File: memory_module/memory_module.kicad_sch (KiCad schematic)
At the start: 93 parts, among them J1 Conn_01x06_Pin, J2 Conn_01x08_Pin, SW1 SW_DIP_x08, SW2 SW_DIP_x08, SW3 SW_DIP_x08, SW4 SW_DIP_x08, SW5 SW_DIP_x08, SW6 SW_DIP_x08, SW7 SW_DIP_x08, SW8 SW_DIP_x08, U1 74HC138, U2 74HC540

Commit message: wip
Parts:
- added D100, D101, D102, D103, D104, D105, D106, D107, D108, D109, D110, D111, D112, D113, D114, D115, D116, D117, D118, D119, D120, D121, D122, D123, D124, D125, D126, D127, D128, D65, D66, D67, D68, D69, D70, D71, D72, D73, D74, D75, D76, D77, D78, D79, D80, D81, D82, D83, D84, D85, D86, D87, D88, D89, D90, D91, D92, D93, D94, D95, D96, D97, D98, D99: 1N4148, Diode_THT:D_DO-35_SOD27_P2.54mm_Vertical_KathodeUp, symbol Diode:1N4148
- added D137, D138, D139, D140, D141, D142, D143, D144: LED, LED_THT:LED_D3.0mm, symbol Device:LED
- added SW10, SW11, SW12, SW13, SW14, SW15, SW16, SW9: SW_DIP_x08, Button_Switch_THT:SW_DIP_SPSTx08_Slide_9.78x22.5mm_W7.62mm_P2.54mm, symbol Switch:SW_DIP_x08
- added U2: 74HC138, TD4_footprint:DIP16_TOS, symbol 74xx:74HC138
- D1, D10, D11, D12, D13, D14, D15, D16, D17, D18, D19, D2, D20, D21, D22, D23, D24, D25, D26, D27, D28, D29, D3, D30, D31, D32, D33, D34, D35, D36, D37, D38, D39, D4, D40, D41, D42, D43, D44, D45, D46, D47, D48, D49, D5, D50, D51, D52, D53, D54, D55, D56, D57, D58, D59, D6, D60, D61, D62, D63, D64, D7, D8, D9: footprint Diode_THT:D_DO-35_SOD27_P7.62mm_Horizontal -> Diode_THT:D_DO-35_SOD27_P2.54mm_Vertical_KathodeUp
- renumbered D65 to D129, D66 to D130, D67 to D131, D68 to D132, D69 to D133, D70 to D134, D71 to D135, D72 to D136, U2 to U3
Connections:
- net +5V: now also U2.16 (VCC)
- net A0: now also U2.1 (A0)
- net A1: now also U2.2 (A1)
- net A2: now also U2.3 (A2)
- net GND: now also U2.5 (~{E1}), U2.6 (E2), U2.8 (GND); no longer J1.4 (Pin_4), U1.5 (~{E1}), U1.6 (E2)
- net at D129.2 (A), D130.2 (A), D131.2 (A)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: now also D137.2 (A), D138.2 (A), D139.2 (A), D140.2 (A), D141.2 (A), D142.2 (A), D143.2 (A), D144.2 (A)
- net at R1.1, SW1.16, SW2.16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: now also SW10.16, SW11.16, SW12.16, SW13.16, SW14.16, SW15.16, SW16.16, SW9.16
- net at R3.1, SW1.14, SW2.14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: now also SW10.14, SW11.14, SW12.14, SW13.14, SW14.14, SW15.14, SW16.14, SW9.14
- net at R6.1, SW1.11, SW2.11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: now also SW10.11, SW11.11, SW12.11, SW13.11, SW14.11, SW15.11, SW16.11, SW9.11
- net at R2.1, SW1.15, SW2.15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: now also SW10.15, SW11.15, SW12.15, SW13.15, SW14.15, SW15.15, SW16.15, SW9.15
- net at R7.1, SW1.10, SW2.10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: now also SW10.10, SW11.10, SW12.10, SW13.10, SW14.10, SW15.10, SW16.10, SW9.10
- net at R5.1, SW1.12, SW2.12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: now also SW10.12, SW11.12, SW12.12, SW13.12, SW14.12, SW15.12, SW16.12, SW9.12
- net at R4.1, SW1.13, SW2.13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: now also SW10.13, SW11.13, SW12.13, SW13.13, SW14.13, SW15.13, SW16.13, SW9.13
- net at R8.1, SW1.9, SW2.9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: now also SW10.9, SW11.9, SW12.9, SW13.9, SW14.9, SW15.9, SW16.9, SW9.9
- new net: D100.1 (K), D101.1 (K), D102.1 (K), D103.1 (K), D104.1 (K), D97.1 (K), D98.1 (K), D99.1 (K)
- new net: D98.2 (A), SW13.2
- new net: D121.2 (A), SW16.1
- new net: D122.2 (A), SW16.2
- new net: D123.2 (A), SW16.3
- new net: D124.2 (A), SW16.4
- new net: D125.2 (A), SW16.5
- new net: D126.2 (A), SW16.6
- new net: D127.2 (A), SW16.7
- new net: D128.2 (A), SW16.8
- new net: D73.1 (K), D74.1 (K), D75.1 (K), D76.1 (K), D77.1 (K), D78.1 (K), D79.1 (K), D80.1 (K)
- new net: D74.2 (A), SW10.2
- new net: D105.1 (K), D106.1 (K), D107.1 (K), D108.1 (K), D109.1 (K), D110.1 (K), D111.1 (K), D112.1 (K)
- new net: D112.2 (A), SW14.8
- new net: D78.2 (A), SW10.6
- new net: D65.2 (A), SW9.1
- new net: D66.2 (A), SW9.2
- new net: D67.2 (A), SW9.3
- new net: D68.2 (A), SW9.4
- new net: D69.2 (A), SW9.5
- new net: D70.2 (A), SW9.6
- new net: D71.2 (A), SW9.7
- new net: D72.2 (A), SW9.8
- new net: D65.1 (K), D66.1 (K), D67.1 (K), D68.1 (K), D69.1 (K), D70.1 (K), D71.1 (K), D72.1 (K)
- new net: D75.2 (A), SW10.3
- new net: D138.1 (K), U2.14 (~{Y1})
- new net: D121.1 (K), D122.1 (K), D123.1 (K), D124.1 (K), D125.1 (K), D126.1 (K), D127.1 (K), D128.1 (K)
- new net: D141.1 (K), U2.11 (~{Y4})
- new net: D73.2 (A), SW10.1
- new net: D113.1 (K), D114.1 (K), D115.1 (K), D116.1 (K), D117.1 (K), D118.1 (K), D119.1 (K), D120.1 (K)
- new net: D114.2 (A), SW15.2
- new net: D120.2 (A), SW15.8
- new net: D81.1 (K), D82.1 (K), D83.1 (K), D84.1 (K), D85.1 (K), D86.1 (K), D87.1 (K), D88.1 (K)
- new net: D85.2 (A), SW11.5
- new net: D101.2 (A), SW13.5
- new net: D84.2 (A), SW11.4
- new net: D89.1 (K), D90.1 (K), D91.1 (K), D92.1 (K), D93.1 (K), D94.1 (K), D95.1 (K), D96.1 (K)
- new net: D90.2 (A), SW12.2
- new net: D81.2 (A), SW11.1
- new net: D82.2 (A), SW11.2
- new net: D83.2 (A), SW11.3
- new net: D86.2 (A), SW11.6
- new net: D87.2 (A), SW11.7
- new net: D88.2 (A), SW11.8
- new net: D108.2 (A), SW14.4
- new net: D117.2 (A), SW15.5
- new net: D95.2 (A), SW12.7
- new net: D111.2 (A), SW14.7
- new net: D103.2 (A), SW13.7
- new net: D107.2 (A), SW14.3
- new net: D105.2 (A), SW14.1
- new net: D106.2 (A), SW14.2
- new net: D109.2 (A), SW14.5
- new net: D110.2 (A), SW14.6
- new net: D139.1 (K), U2.13 (~{Y2})
- new net: D91.2 (A), SW12.3
- new net: D119.2 (A), SW15.7
- new net: D77.2 (A), SW10.5
- new net: D93.2 (A), SW12.5
- new net: D97.2 (A), SW13.1
- new net: D99.2 (A), SW13.3
- new net: D100.2 (A), SW13.4
- new net: D102.2 (A), SW13.6
- new net: D104.2 (A), SW13.8
- new net: D137.1 (K), U2.15 (~{Y0})
- new net: D144.1 (K), U2.7 (~{Y7})
- new net: D115.2 (A), SW15.3
- new net: D89.2 (A), SW12.1
- new net: D92.2 (A), SW12.4
- new net: D94.2 (A), SW12.6
- new net: D96.2 (A), SW12.8
- new net: D142.1 (K), U2.10 (~{Y5})
- new net: D140.1 (K), U2.12 (~{Y3})
- new net: D143.1 (K), U2.9 (~{Y6})
- new net: D76.2 (A), SW10.4
- new net: D113.2 (A), SW15.1
- new net: D116.2 (A), SW15.4
- new net: D118.2 (A), SW15.6
- new net: D79.2 (A), SW10.7
- new net: D80.2 (A), SW10.8
- new net A3: J1.4 (Pin_4), U1.5 (~{E1}), U1.6 (E2), U2.4 (~{E0})
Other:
- moved on the sheet: D1, D10, D11, D12, D129, D13, D130, D131, D132, D133, D134, D135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

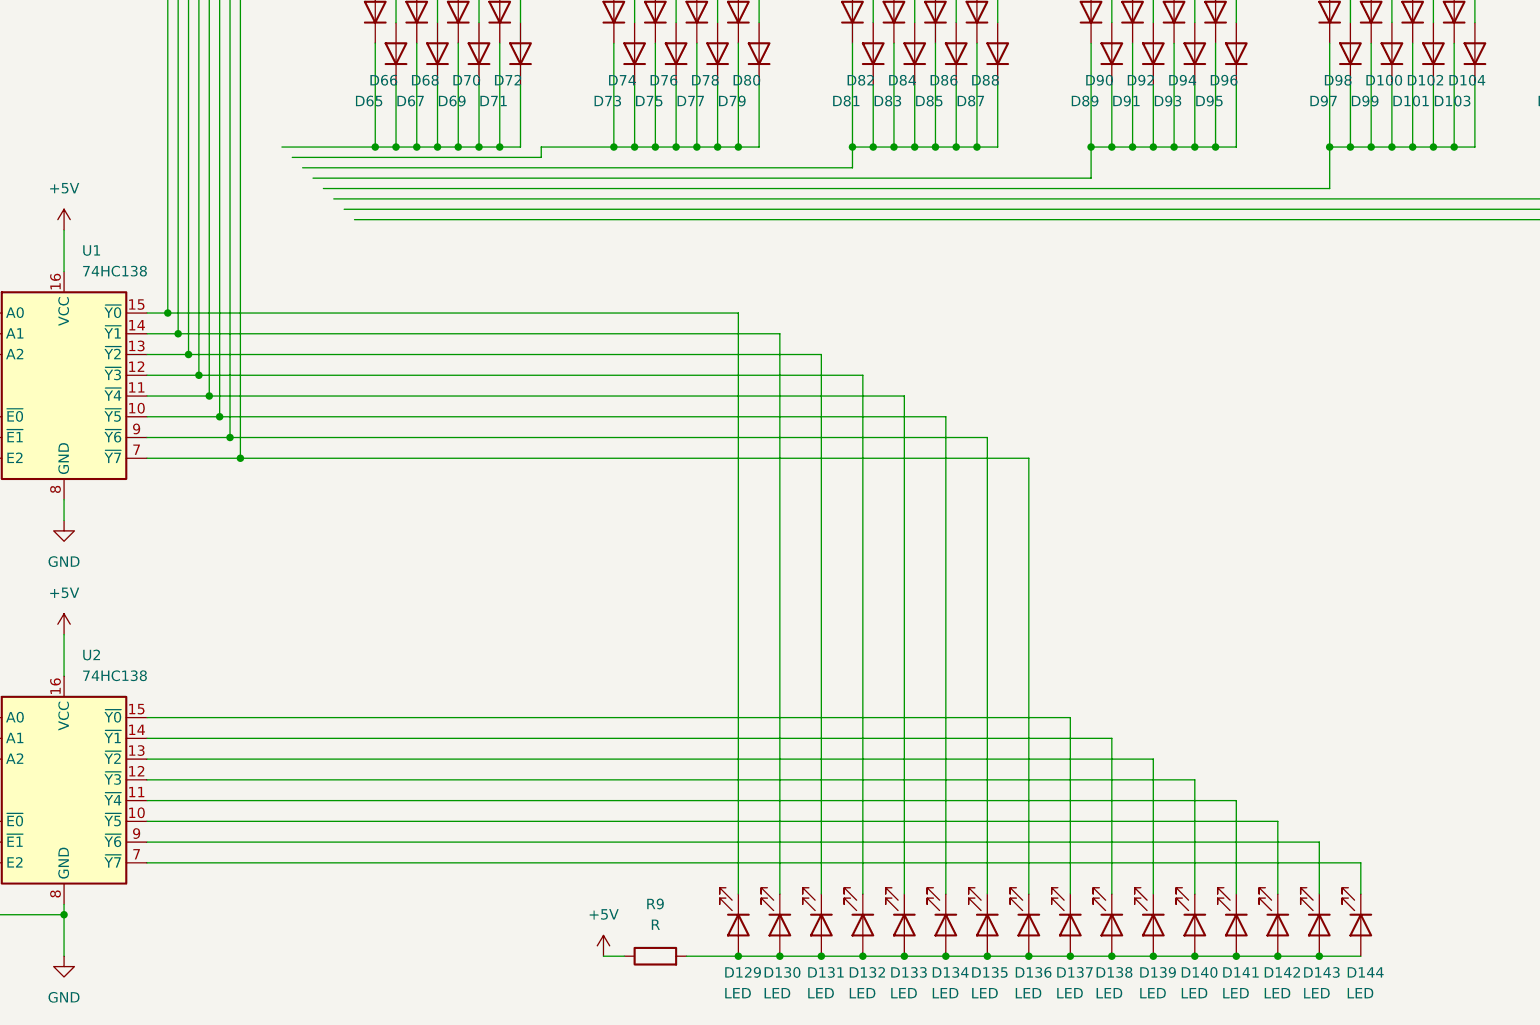
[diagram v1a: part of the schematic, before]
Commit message: wip
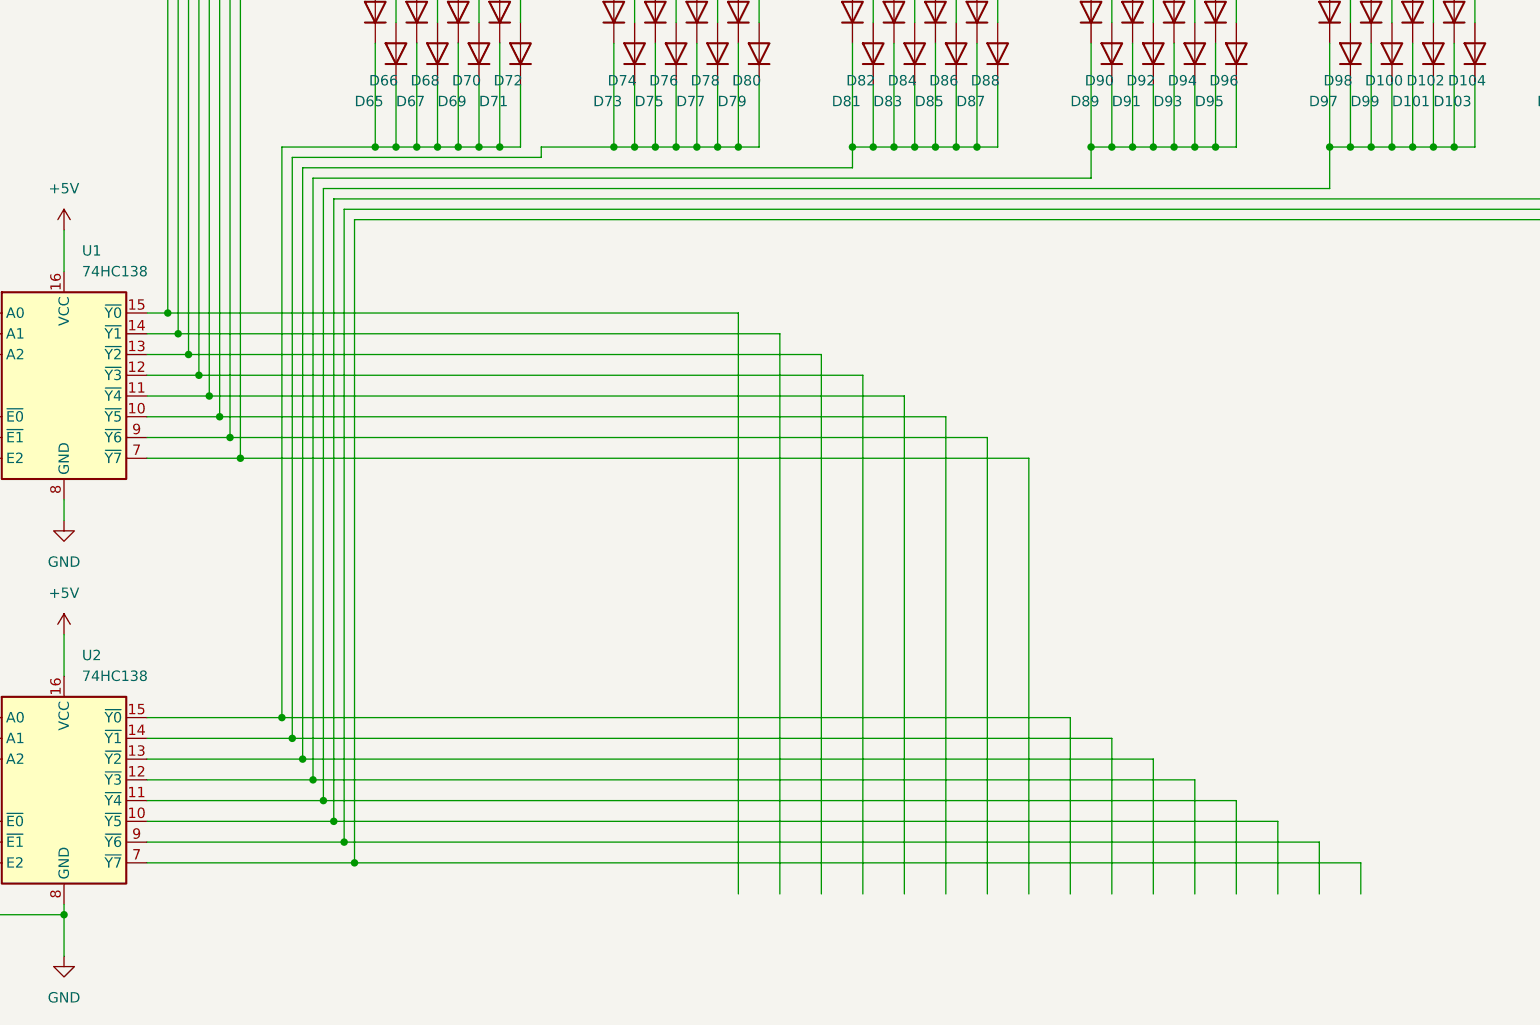
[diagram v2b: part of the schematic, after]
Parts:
- removed D129, D130, D131, D132, D133, D134, D135, D136, D137, D138, D139, D140, D141, D142, D143, D144: LED, LED_THT:LED_D3.0mm, symbol Device:LED
- removed R9: R, Resistor_THT:R_Axial_DIN0207_L6.3mm_D2.5mm_P10.16mm_Horizontal, symbol Device:R
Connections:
- net at D100.1 (K), D101.1 (K), D102.1 (K)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: now also U2.11 (~{Y4})
- net at D73.1 (K), D74.1 (K), D75.1 (K)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: now also U2.14 (~{Y1})
- net at D105.1 (K), D106.1 (K), D107.1 (K)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: now also U2.10 (~{Y5})
- net at D65.1 (K), D66.1 (K), D67.1 (K)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: now also U2.15 (~{Y0})
- net at D121.1 (K), D122.1 (K), D123.1 (K)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: now also U2.7 (~{Y7})
- net at D113.1 (K), D114.1 (K), D115.1 (K)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: now also U2.9 (~{Y6})
- net at D81.1 (K), D82.1 (K), D83.1 (K)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: now also U2.13 (~{Y2})
- net at D89.1 (K), D90.1 (K), D91.1 (K)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: now also U2.12 (~{Y3})

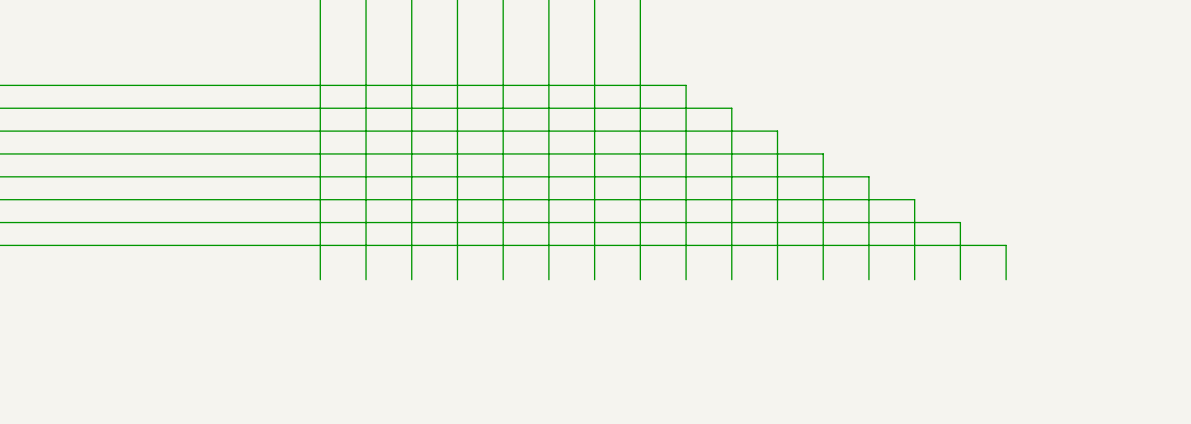
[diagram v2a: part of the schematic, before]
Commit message: とりあえず配線した、美しくはない
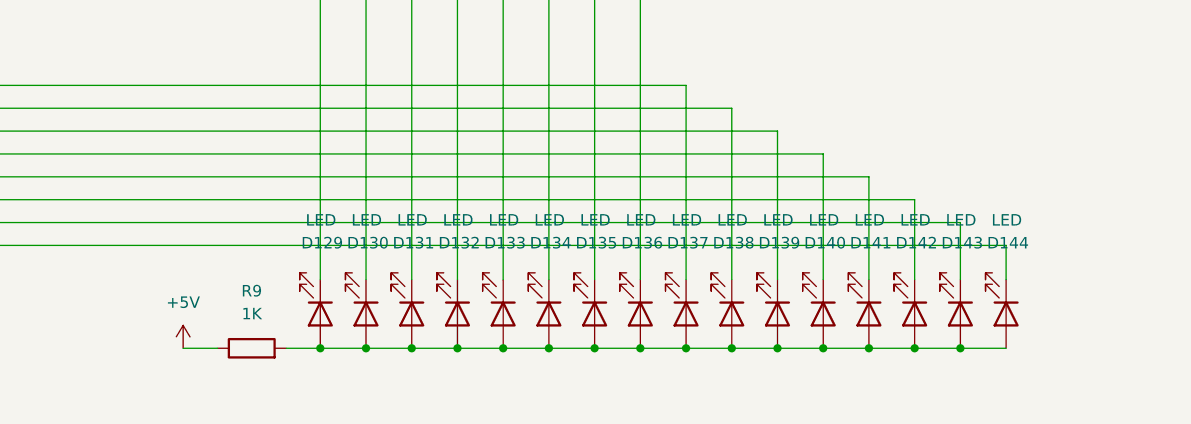
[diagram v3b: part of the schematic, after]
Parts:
- added D129, D130, D131, D132, D133, D134, D135, D136, D137, D138, D139, D140, D141, D142, D143, D144: LED, LED_SMD:LED_1206_3216Metric_Pad1.42x1.75mm_HandSolder, symbol Device:LED
- added R9: 1K, Resistor_THT:R_Axial_DIN0207_L6.3mm_D2.5mm_P2.54mm_Vertical, symbol Device:R
- R1, R2: value R -> 10K; footprint Resistor_THT:R_Axial_DIN0207_L6.3mm_D2.5mm_P10.16mm_Horizontal -> Resistor_THT:R_Axial_DIN0207_L6.3mm_D2.5mm_P2.54mm_Vertical
- R3, R4, R5, R6, R7, R8: footprint Resistor_THT:R_Axial_DIN0207_L6.3mm_D2.5mm_P10.16mm_Horizontal -> Resistor_THT:R_Axial_DIN0207_L6.3mm_D2.5mm_P2.54mm_Vertical
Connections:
- net +5V: now also R9.1
- net at D100.1 (K), D101.1 (K), D102.1 (K)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: now also D141.1 (K)
- net at D73.1 (K), D74.1 (K), D75.1 (K)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: now also D138.1 (K)
- net at D105.1 (K), D106.1 (K), D107.1 (K)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: now also D142.1 (K)
- net at D10.1 (K), D11.1 (K), D12.1 (K)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: now also D130.1 (K)
- net at D49.1 (K), D50.1 (K), D51.1 (K)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: now also D135.1 (K)
- net at D25.1 (K), D26.1 (K), D27.1 (K)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: now also D132.1 (K)
- net at D65.1 (K), D66.1 (K), D67.1 (K)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: now also D137.1 (K)
- net at D121.1 (K), D122.1 (K), D123.1 (K)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: now also D144.1 (K)
- net at D17.1 (K), D18.1 (K), D19.1 (K)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: now also D131.1 (K)
- net at D113.1 (K), D114.1 (K), D115.1 (K)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: now also D143.1 (K)
- net at D81.1 (K), D82.1 (K), D83.1 (K)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: now also D139.1 (K)
- net at D1.1 (K), D2.1 (K), D3.1 (K)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: now also D129.1 (K)
- net at D57.1 (K), D58.1 (K), D59.1 (K)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: now also D136.1 (K)
- net at D33.1 (K), D34.1 (K), D35.1 (K)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: now also D133.1 (K)
- net at D89.1 (K), D90.1 (K), D91.1 (K)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: now also D140.1 (K)
- net at D41.1 (K), D42.1 (K), D43.1 (K)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: now also D134.1 (K)
- new net: D129.2 (A), D130.2 (A), D131.2 (A), D132.2 (A), D133.2 (A), D134.2 (A), D135.2 (A), D136.2 (A), D137.2 (A), D138.2 (A), D139.2 (A), D140.2 (A), D141.2 (A), D142.2 (A), D143.2 (A), D144.2 (A), R9.2
